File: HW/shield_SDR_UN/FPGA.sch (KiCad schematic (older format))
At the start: 41 parts

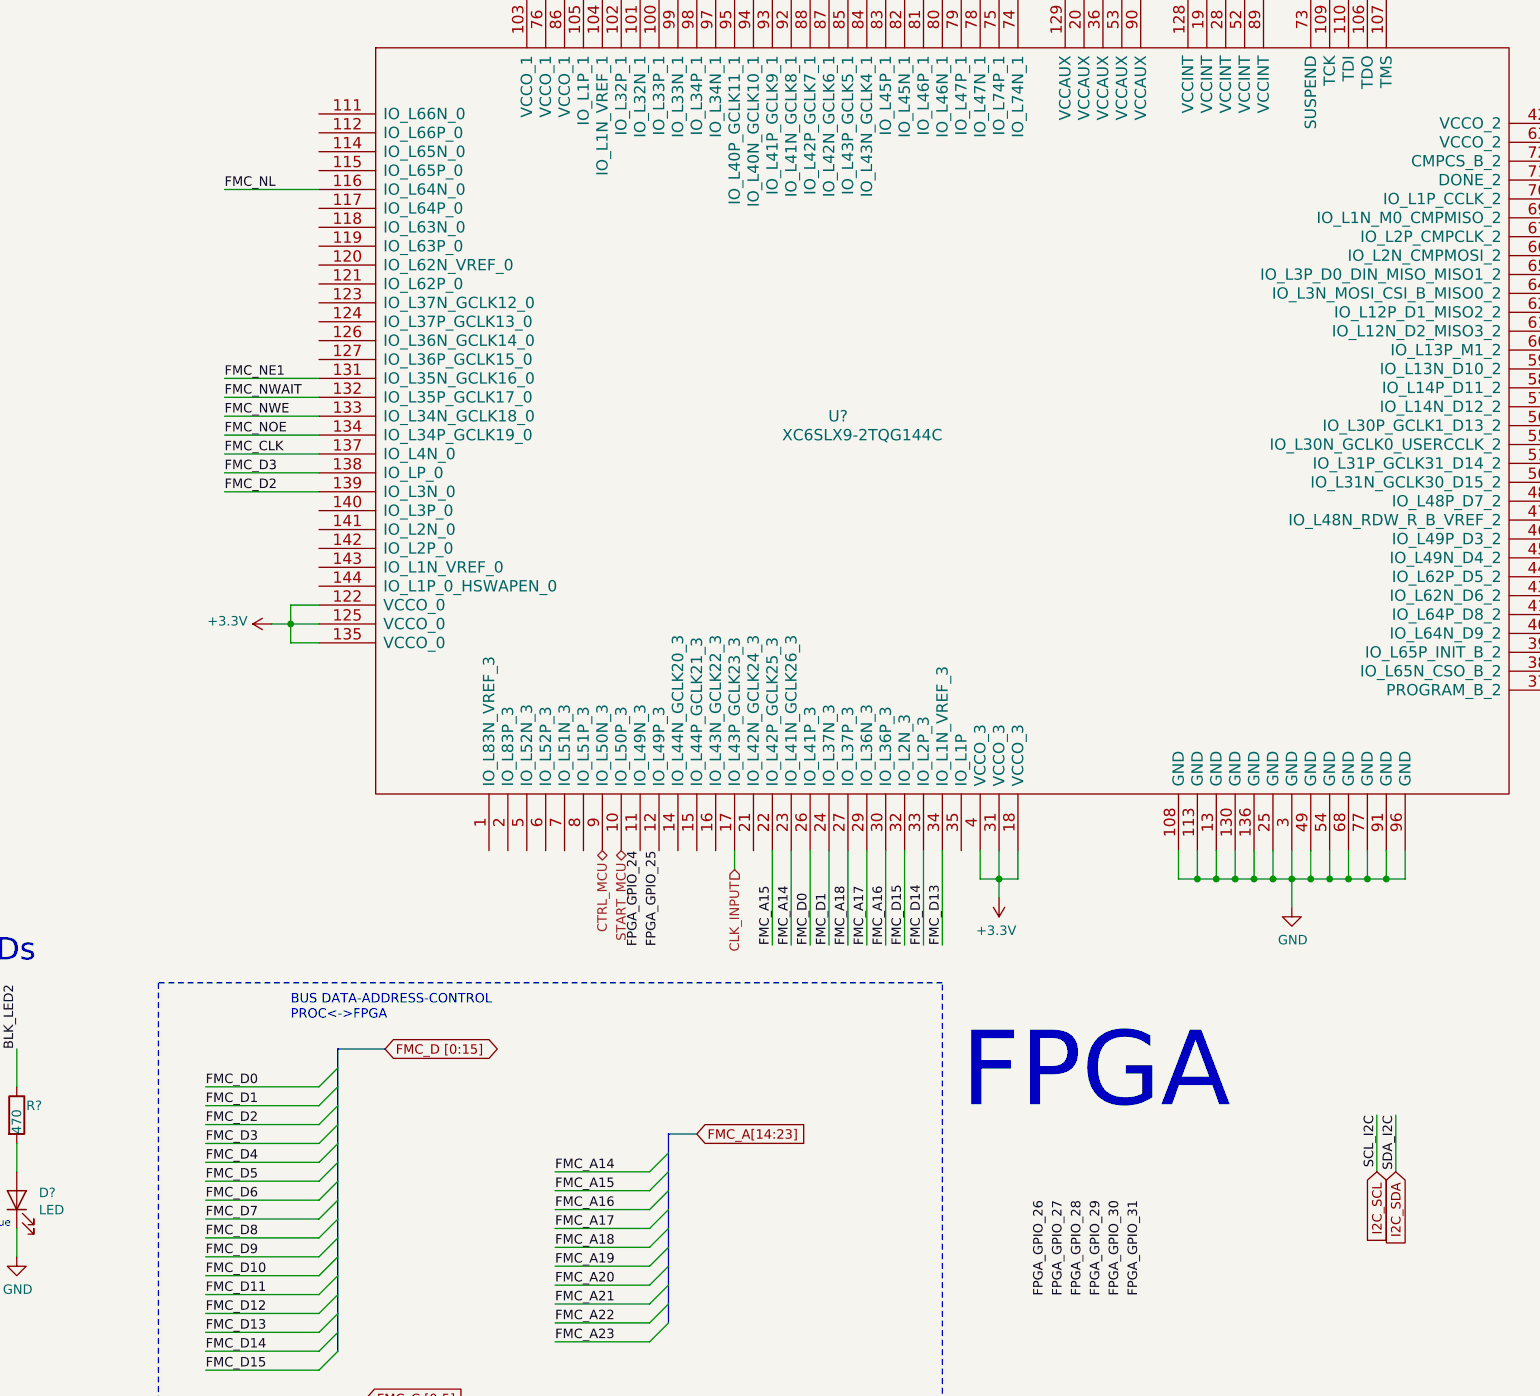
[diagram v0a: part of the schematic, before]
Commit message: i2c_complete
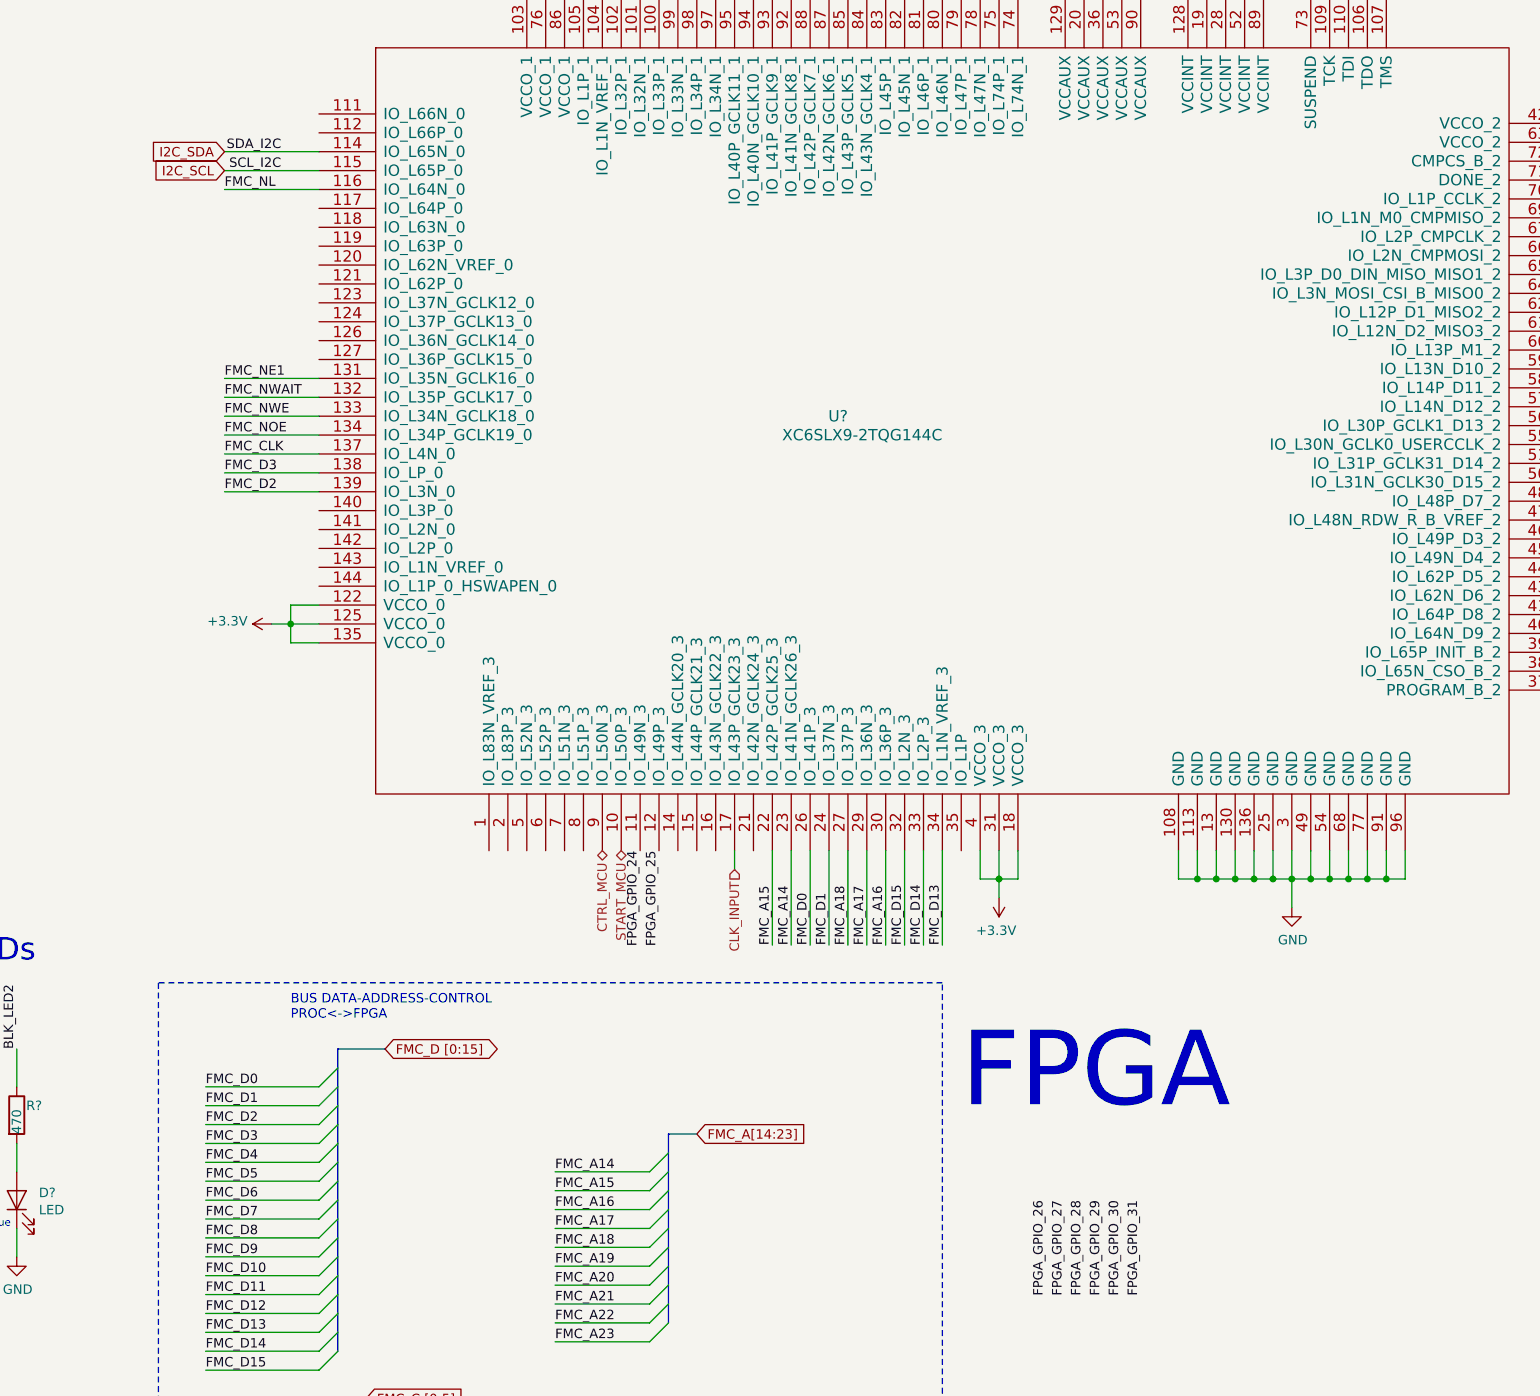
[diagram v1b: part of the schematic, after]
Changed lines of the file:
@@
 Text HLabel 7100 6650 3    50   BiDi ~ 0
 CTRL_MCU
-Text Label 11200 8050 3    50   ~ 0
+Text Label 5400 3050 2    50   ~ 0
 SCL_I2C
-Text Label 11300 8050 3    50   ~ 0
+Text Label 5400 2950 2    50   ~ 0
 SDA_I2C
 Text Label 3450 7700 1    50   ~ 0
 BLK_LED1
-Wire Wire Line
-	11300 8050 11300 8350
-Wire Wire Line
-	11200 8050 11200 8350
 $Comp
 L Connector_Generic:Conn_02x18_Counter_Clockwise J?
@@
 Text Notes 1550 7250 0    118  ~ 0
 GPIO Pins
-Text GLabel 11200 8350 3    50   Input ~ 0
-I2C_SCL
-Text GLabel 11300 8350 3    50   Input ~ 0
-I2C_SDA
 $Comp
 L power:+3.3V #PWR0154
@@
 Text Label 8800 7150 1    50   ~ 0
 FMC_D14
+Text GLabel 5100 3050 0    50   Input ~ 0
+I2C_SCL
+Text GLabel 5100 2950 0    50   Input ~ 0
+I2C_SDA
+Wire Wire Line
+	5100 2950 5600 2950
+Wire Wire Line
+	5100 3050 5600 3050
 Wire Bus Line
 	5700 9550 5700 10150

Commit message: Schematic finished
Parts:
- removed D?: LED, LED_SMD:LED_0805_2012Metric_Pad1.15x1.40mm_HandSolder, symbol Device:LED
- removed D?: LED, LED_SMD:LED_0603_1608Metric_Pad1.05x0.95mm_HandSolder, symbol Device:LED
- removed J?: Conn_02x18_Counter_Clockwise, symbol Connector_Generic:Conn_02x18_Counter_Clockwise
- removed R? (x2): 220, Resistor_SMD:R_0603_1608Metric_Pad1.05x0.95mm_HandSolder, symbol Device:R
- removed R?: 4.7k, Resistor_SMD:R_0603_1608Metric_Pad1.05x0.95mm_HandSolder, symbol Device:R
- removed SW?: SW_Push, SWITCH_FSM1LPA, symbol FSM1LPTR:FSM1LPTR
- added C85, C86: 100nF, Capacitor_SMD:C_0603_1608Metric_Pad1.05x0.95mm_HandSolder, symbol Device:C
- added D3, D4: LED, LED_SMD:LED_0805_2012Metric_Pad1.15x1.40mm_HandSolder, symbol Device:LED
- added J1: Conn_02x09_Odd_Even, Connector_PinHeader_2.54mm:PinHeader_2x09_P2.54mm_Vertical, symbol Connector_Generic:Conn_02x09_Odd_Even
- added J2: Conn_02x08_Odd_Even, Connector_PinHeader_2.54mm:PinHeader_2x08_P2.54mm_Vertical, symbol Connector_Generic:Conn_02x08_Odd_Even
- added R24, R25, R26, R27, R28, R29, R30, R33, R34, R35, R36, R37, R38, R39, R40, R41, R42, R43, R44, R45, R46, R47, R48: 200, Resistor_SMD:R_0603_1608Metric_Pad1.05x0.95mm_HandSolder, symbol Device:R
- added R49, R50: 10k, Resistor_SMD:R_0603_1608Metric_Pad1.05x0.95mm_HandSolder, symbol Device:R
- added R51, R52: 470, Resistor_SMD:R_0603_1608Metric_Pad1.05x0.95mm_HandSolder, symbol Device:R
- added R53: 4.7k, Resistor_SMD:R_0603_1608Metric_Pad1.05x0.95mm_HandSolder, symbol Device:R
- added S1, S2, S3: TL1014BF160QG, lib:TL1014BF160QG, symbol TL1014BF160QG:TL1014BF160QG
- gave numbers to parts that had none: 34
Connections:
- net labels added: BTN1, BTN2, FMC_NBL0, FMC_NBL1
- net labels removed: CLK_INPUT, CTRL_MCU, FMC_A[14:23], FMC_C [0:5], FMC_D [0:15], FPGA_GPIO_23, FPGA_GPIO_24, FPGA_GPIO_25, FPGA_GPIO_26, FPGA_GPIO_27, FPGA_GPIO_28, FPGA_GPIO_29, FPGA_GPIO_30, FPGA_GPIO_31, START_MCU
- wire segments 350 -> 431
- no-connect marks 1 -> 19
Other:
- note added: "Buttons"
- moved on the sheet: C58, C62, C66, C70, C74, D2, R31, R32
